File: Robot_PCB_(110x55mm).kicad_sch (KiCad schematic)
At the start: 20 parts, among them U1 L293, U2 SW_DPDT_XLX, U3 AMS1117-5.0, U5 MFRC522 37.5x25mm

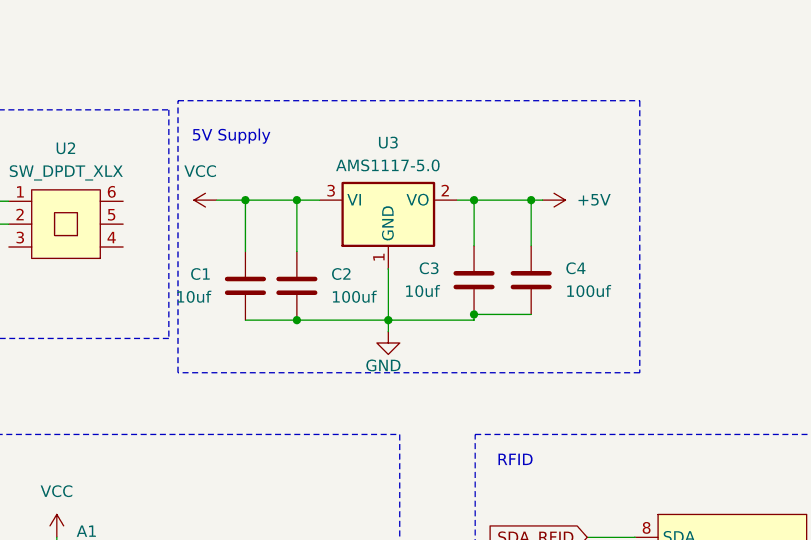
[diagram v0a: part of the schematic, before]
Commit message: update
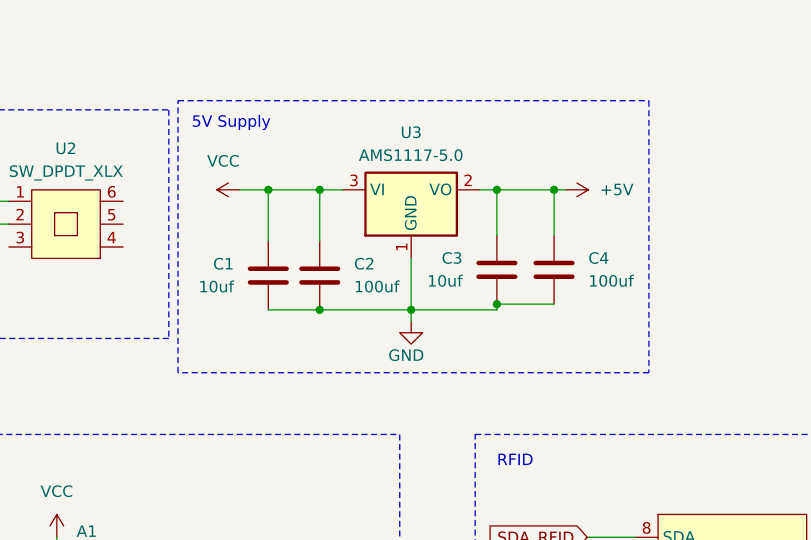
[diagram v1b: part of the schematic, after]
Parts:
- C5, C6: footprint Capacitor_SMD:C_0603_1608Metric -> Capacitor_SMD:C_0805_2012Metric_Pad1.18x1.45mm_HandSolder
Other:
- moved on the sheet: C1, C2, C3, C4, U3

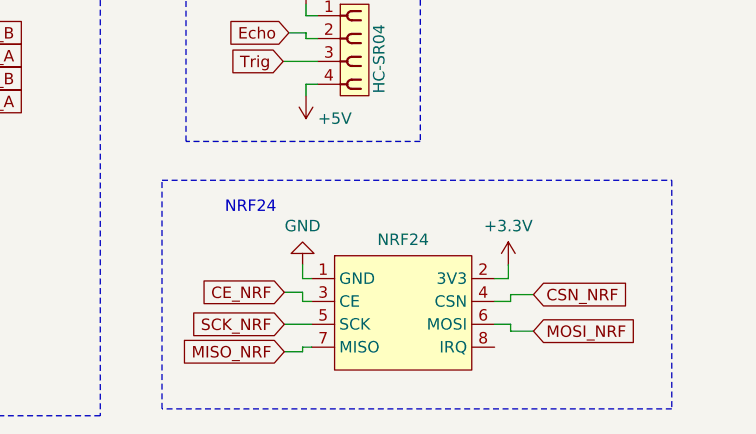
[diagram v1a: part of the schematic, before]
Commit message: Update
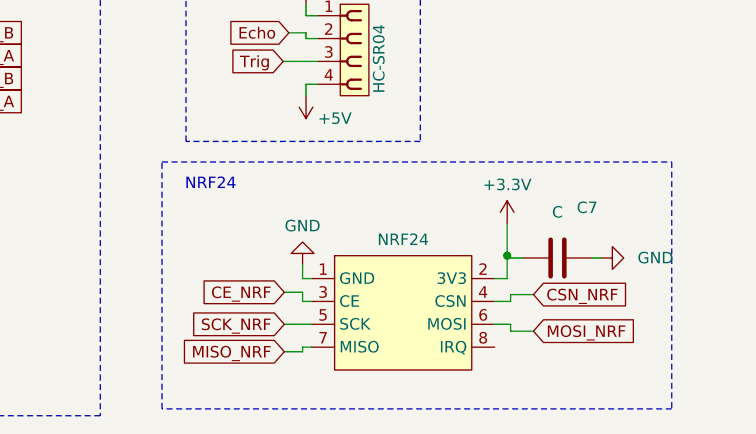
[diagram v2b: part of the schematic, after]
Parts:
- added C7: C, Capacitor_SMD:C_0805_2012Metric_Pad1.18x1.45mm_HandSolder, symbol Device:C
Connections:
- net +3.3V: now also C7.1
- net GND: now also C7.2
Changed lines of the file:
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@@
   (junction (at 175.895 32.512) (diameter 0) (color 0 0 0 0)
   )
+  (junction (at 235.712 137.16) (diameter 0) (color 0 0 0 0)
+  )
   (junction (at 201.295 32.512) (diameter 0) (color 0 0 0 0)
   )
@@
     (stroke (width 0) (type default))
   )
+  (wire (pts (xy 235.712 133.604) (xy 235.712 137.16))
+    (stroke (width 0) (type default))
+  )
+  (wire (pts (xy 245.11 137.414) (xy 246.126 137.414))
+    (stroke (width 0) (type default))
+  )
   (wire (pts (xy 51.308 98.298) (xy 43.815 98.298))
     (stroke (width 0) (type default))
@@
     (stroke (width 0) (type default))
   )
+  (wire (pts (xy 237.49 137.414) (xy 235.966 137.414))
+    (stroke (width 0) (type default))
+  )
   (wire (pts (xy 170.18 114.935) (xy 172.72 114.935))
     (stroke (width 0) (type default))
@@
     (stroke (width 0) (type default))
   )
-  (wire (pts (xy 235.839 139.7) (xy 235.839 138.176))
+  (wire (pts (xy 235.712 139.7) (xy 235.712 137.16))
     (stroke (width 0) (type default))
   )
@@
     (stroke (width 0) (type default))
   )
-  (wire (pts (xy 234.315 139.7) (xy 235.839 139.7))
+  (wire (pts (xy 234.315 139.7) (xy 235.712 139.7))
     (stroke (width 0) (type default))
   )
@@
     (stroke (width 0) (type default))
   )
+  (wire (pts (xy 235.966 137.414) (xy 235.966 137.16))
+    (stroke (width 0) (type default))
+  )
   (wire (pts (xy 201.295 32.512) (xy 201.295 37.592))
     (stroke (width 0) (type default))
@@
   )
   (wire (pts (xy 181.61 32.512) (xy 184.15 32.512))
+    (stroke (width 0) (type default))
+  )
+  (wire (pts (xy 235.966 137.16) (xy 235.712 137.16))
     (stroke (width 0) (type default))
   )
@@
     (fill (type none))
   )
-  (rectangle (start 197.358 128.778) (end 254 154.178)
+  (rectangle (start 197.358 126.746) (end 254 154.178)
     (stroke (width 0) (type dash))
     (fill (type none))
@@
     (fill (type none))
   )
-  (text "NRF24" (at 204.343 132.588 0)
+  (text "NRF24" (at 199.898 130.048 0)
     (effects (font (size 1.27 1.27)) (justify left bottom))
   )
@@
         (path "/5740c1d8-40a5-48a4-b0ff-1fed8540b5f6"
           (reference "#PWR05") (unit 1)
+        )
+      )
+    )
+  )
+  (symbol (lib_id "Device:C") (at 241.3 137.414 90) (unit 1)
+    (in_bom yes) (on_board yes) (dnp no)
+    (property "Reference" "C7" (at 244.602 131.826 90)
+      (effects (font (size 1.27 1.27)))
+    )
+    (property "Value" "C" (at 241.3 132.334 90)
+      (effects (font (size 1.27 1.27)))
+    )
+    (property "Footprint" "Capacitor_SMD:C_0805_2012Metric_Pad1.18x1.45mm_HandSolder" (at 245.11 136.4488 0)
+      (effects (font (size 1.27 1.27)) hide)
+    )
+    (property "Datasheet" "~" (at 241.3 137.414 0)
+      (effects (font (size 1.27 1.27)) hide)
+    )
+    (pin "1")
+    (pin "2")
+    (instances
+      (project "Robot_PCB_(110x55mm)"
+        (path "/5740c1d8-40a5-48a4-b0ff-1fed8540b5f6"
+          (reference "C7") (unit 1)
         )
       )
@@
     )
   )
-  (symbol (lib_id "power:+3.3V") (at 235.839 138.176 0) (unit 1)
-    (in_bom yes) (on_board yes) (dnp no) (fields_autoplaced)
-    (property "Reference" "#PWR027" (at 235.839 141.986 0)
-      (effects (font (size 1.27 1.27)) hide)
-    )
-    (property "Value" "+3.3V" (at 235.839 133.858 0)
-      (effects (font (size 1.27 1.27)))
-    )
-    (property "Footprint" "" (at 235.839 138.176 0)
-      (effects (font (size 1.27 1.27)) hide)
-    )
-    (property "Datasheet" "" (at 235.839 138.176 0)
+  (symbol (lib_id "power:+3.3V") (at 235.712 133.604 0) (unit 1)
+    (in_bom yes) (on_board yes) (dnp no) (fields_autoplaced)
+    (property "Reference" "#PWR027" (at 235.712 137.414 0)
+      (effects (font (size 1.27 1.27)) hide)
+    )
+    (property "Value" "+3.3V" (at 235.712 129.286 0)
+      (effects (font (size 1.27 1.27)))
+    )
+    (property "Footprint" "" (at 235.712 133.604 0)
+      (effects (font (size 1.27 1.27)) hide)
+    )
+    (property "Datasheet" "" (at 235.712 133.604 0)
       (effects (font (size 1.27 1.27)) hide)
     )
@@
         )
       )
+    )
+  )
+  (symbol (lib_id "power:GND") (at 246.126 137.414 90) (unit 1)
+    (in_bom yes) (on_board yes) (dnp no) (fields_autoplaced)
+    (property "Reference" "#PWR029" (at 252.476 137.414 0)
+      (effects (font (size 1.27 1.27)) hide)
+    )
+    (property "Value" "GND" (at 250.19 137.414 90)
+      (effects (font (size 1.27 1.27)) (justify right))
+    )
+    (property "Footprint" "" (at 246.126 137.414 0)
+      (effects (font (size 1.27 1.27)) hide)
+    )
+    (property "Datasheet" "" (at 246.126 137.414 0)
+      (effects (font (size 1.27 1.27)) hide)
+    )
+    (pin "1")
+    (instances
+      (project "Robot_PCB_(110x55mm)"
+        (path "/5740c1d8-40a5-48a4-b0ff-1fed8540b5f6"
+          (reference "#PWR029") (unit 1)
+        )
+      )
